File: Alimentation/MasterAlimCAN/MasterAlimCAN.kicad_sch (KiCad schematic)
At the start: 26 parts, among them J1 Batt, U1 AMS1117-3.3, U2 STM32G474RETx, Y1 16MHz

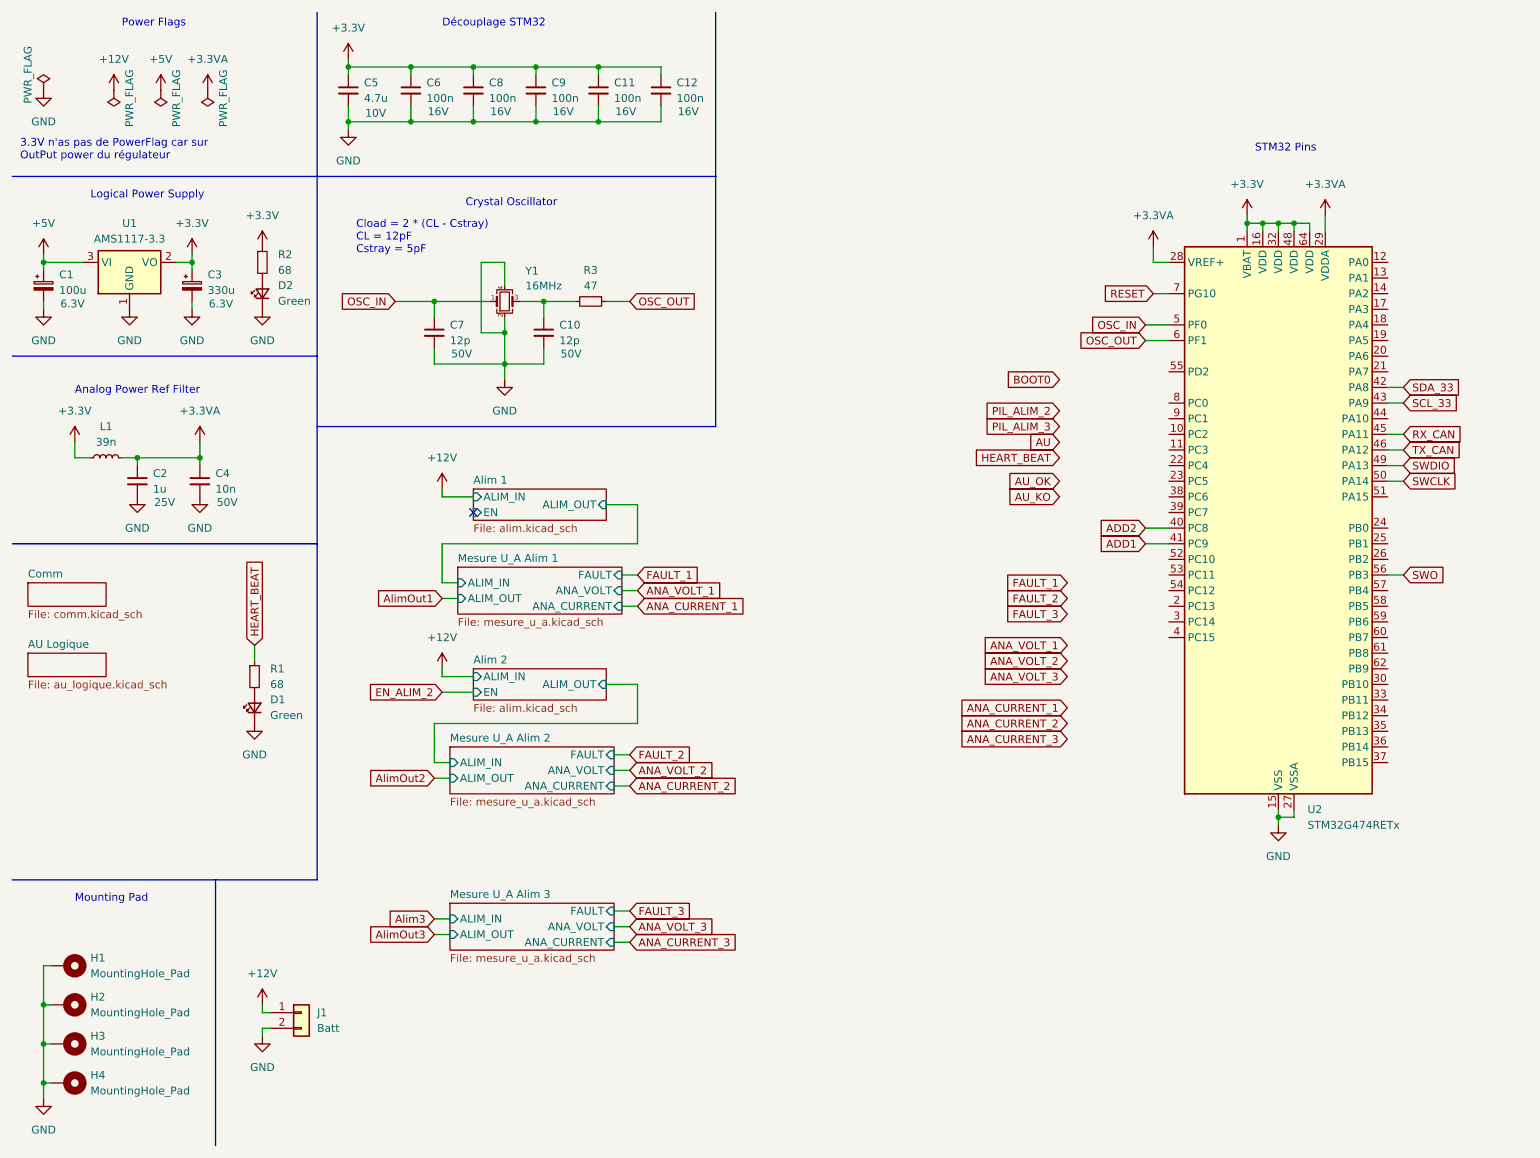
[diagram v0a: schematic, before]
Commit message: Init placement for MasterAlimCAN
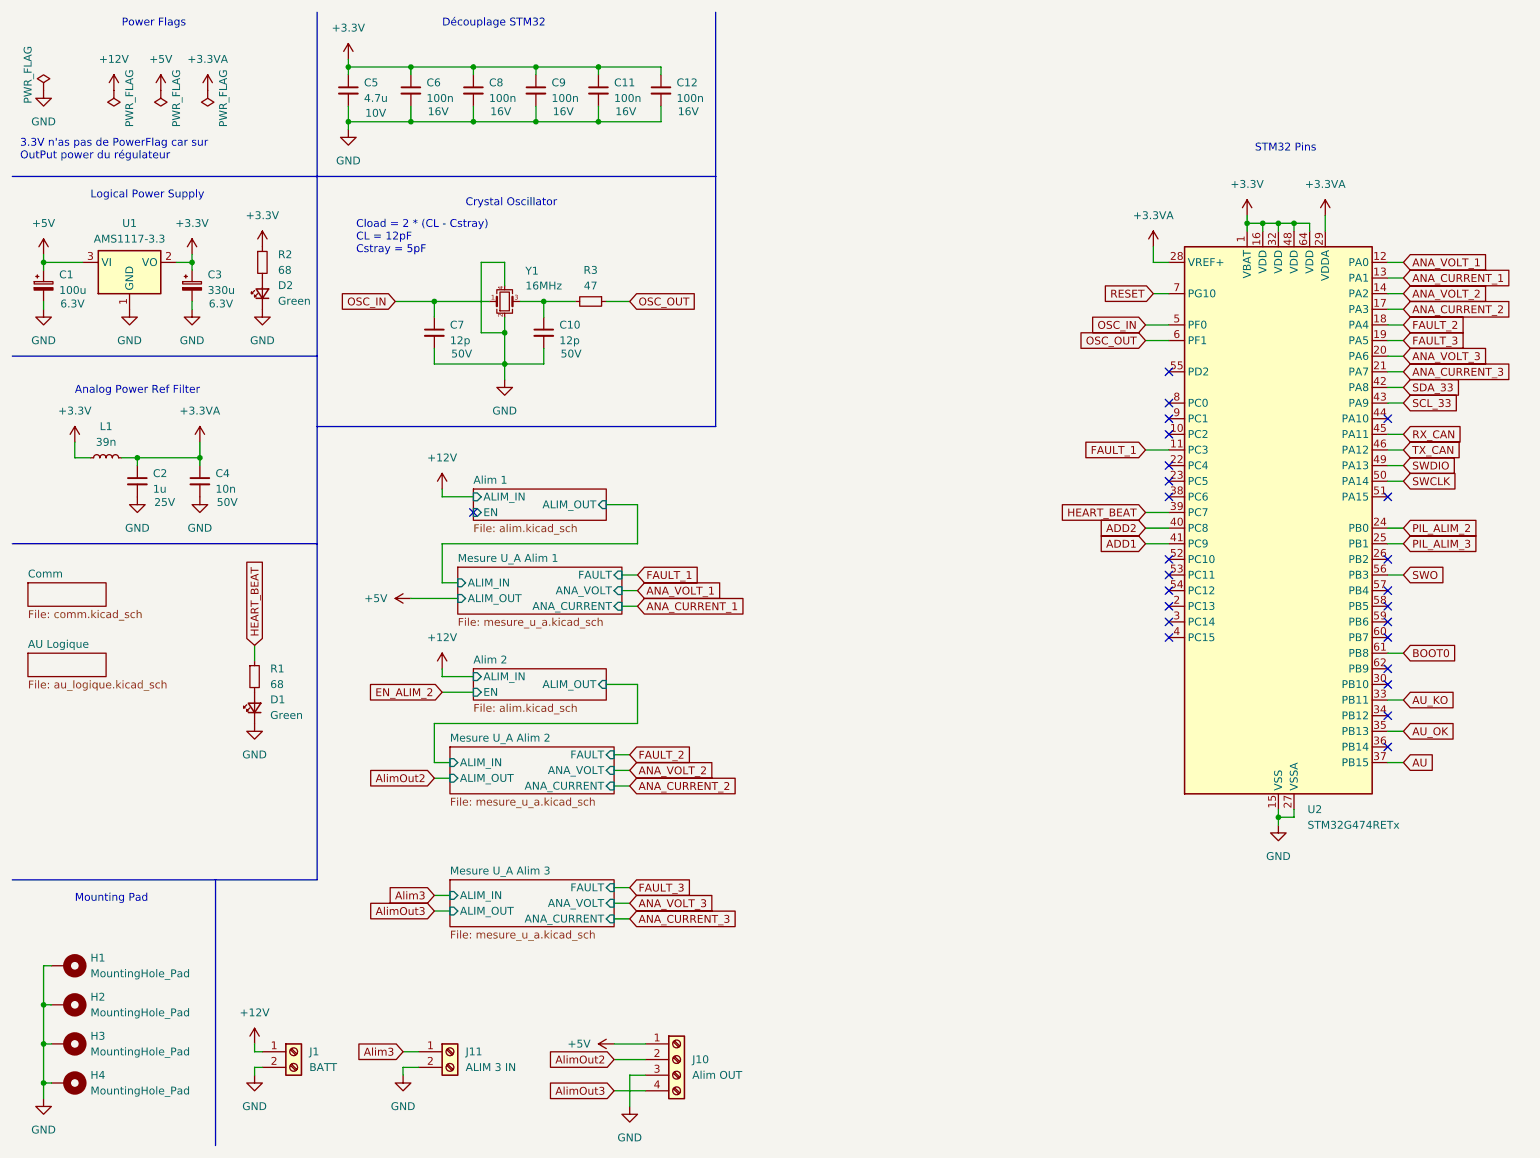
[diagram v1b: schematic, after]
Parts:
- removed J1: Batt, Connector_AMASS:AMASS_XT60-F_1x02_P7.20mm_Vertical, symbol Connector_Generic:Conn_01x02
- added J1: BATT, TerminalBlock_Phoenix:TerminalBlock_Phoenix_MKDS-1,5-2-5.08_1x02_P5.08mm_Horizontal, symbol Connector:Screw_Terminal_01x02
- added J10: Alim OUT, TerminalBlock_Phoenix:TerminalBlock_Phoenix_MKDS-1,5-4-5.08_1x04_P5.08mm_Horizontal, symbol Connector:Screw_Terminal_01x04
- added J11: ALIM 3 IN, TerminalBlock_Phoenix:TerminalBlock_Phoenix_MKDS-1,5-2-5.08_1x02_P5.08mm_Horizontal, symbol Connector:Screw_Terminal_01x02
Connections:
- net +12V: now also J1.1 (Pin_1)
- net +5V: now also J10.1 (Pin_1)
- net ANA_CURRENT_1: now also U2.13 (PA1)
- net ANA_CURRENT_2: now also U2.17 (PA3)
- net ANA_CURRENT_3: now also U2.21 (PA7)
- net ANA_VOLT_1: now also U2.12 (PA0)
- net ANA_VOLT_2: now also U2.14 (PA2)
- net ANA_VOLT_3: now also U2.20 (PA6)
- net AU: now also U2.37 (PB15)
- net AU_KO: now also U2.33 (PB11)
- net AU_OK: now also U2.35 (PB13)
- net Alim3: now also J11.1 (Pin_1)
- net AlimOut2: now also J10.2 (Pin_2)
- net AlimOut3: now also J10.4 (Pin_4)
- net BOOT0: now also U2.61 (PB8)
- net FAULT_1: now also U2.11 (PC3)
- net FAULT_2: now also U2.18 (PA4)
- net FAULT_3: now also U2.19 (PA5)
- net GND: now also J1.2 (Pin_2), J10.3 (Pin_3), J11.2 (Pin_2)
- net HEART_BEAT: now also U2.39 (PC7)
- net PIL_ALIM_2: now also U2.24 (PB0)
- net PIL_ALIM_3: now also U2.25 (PB1)
- no-connect marks 1 -> 25
